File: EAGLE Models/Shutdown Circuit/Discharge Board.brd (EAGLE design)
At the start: 108 x 60 mm, 12 parts, among them U1 G2RL-1-E, U2 G2RL-1-E

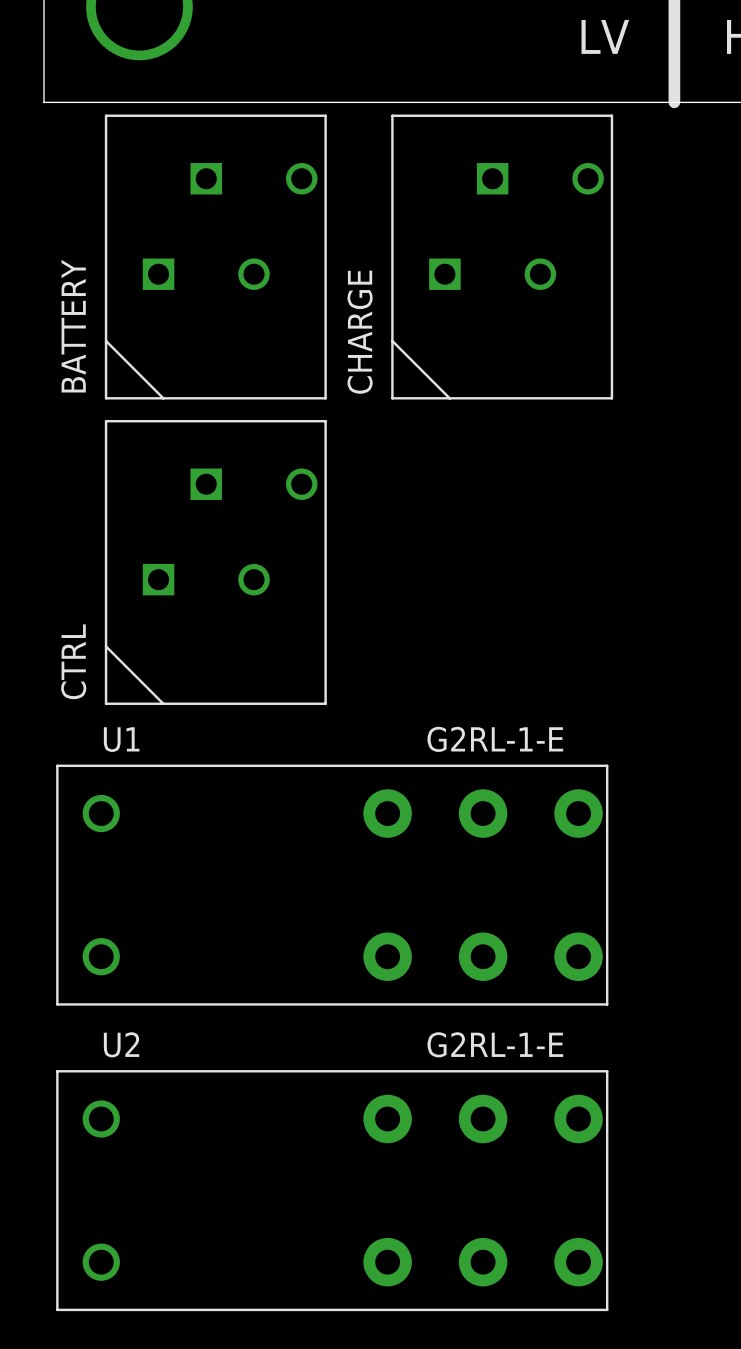
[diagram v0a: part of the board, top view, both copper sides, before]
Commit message: Deleted random parts that got added to the layout
These random parts were not in the schematic so I deleted them.
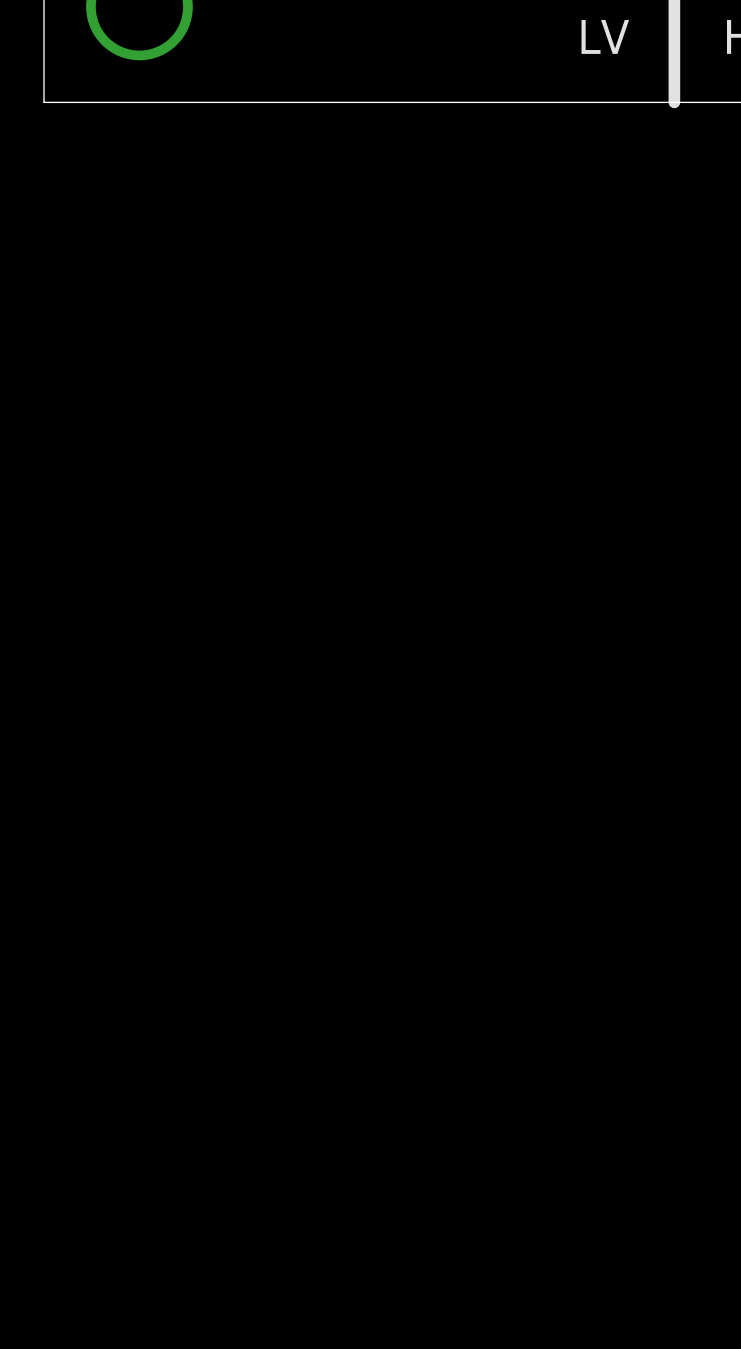
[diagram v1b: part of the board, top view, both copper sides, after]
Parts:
- removed BATTERY, CHARGE, CTRL: CONN_2, formula electric:CONNECTOR_2
- removed U1, U2: G2RL-1-E, formula electric:G2RL-1-E_RELAY
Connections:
- removed net N$1: CTRL.3, CTRL.4, U1.P$8, U2.P$8
- removed net N$12: BATTERY.1, BATTERY.2, U2.P$4, U2.P$5
- removed net N$13: BATTERY.3, BATTERY.4, U1.P$4, U1.P$5
- removed net N$14: CHARGE.1, CHARGE.2, U2.P$3, U2.P$6
- removed net N$15: CHARGE.3, CHARGE.4, U1.P$3, U1.P$6
- removed net N$2: CTRL.1, CTRL.2, U1.P$1, U2.P$1
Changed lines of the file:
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@@
 <?xml version="1.0" encoding="utf-8"?>
 <!DOCTYPE eagle SYSTEM "eagle.dtd">
-<eagle version="7.1.0">
+<eagle version="8.0.1">
 <drawing>
 <settings>
@@
 <element name="R2" library="formula electric" package="VISHAY_FS20W_RES" value="500" x="27" y="42"/>
 <element name="R3" library="formula electric" package="VISHAY_FS20W_RES" value="500" x="80" y="42" rot="R180"/>
-<element name="BATTERY" library="formula electric" package="CONNECTOR_2" value="CONN_2" x="6" y="-9"/>
-<element name="CTRL" library="formula electric" package="CONNECTOR_2" value="CONN_2" x="6" y="-25"/>
-<element name="U2" library="formula electric" package="G2RL-1-E_RELAY" value="G2RL-1-E" x="18" y="-57">
-<attribute name="COIL" value="DC 12" x="-13" y="-10" size="1.778" layer="27" display="off"/>
-</element>
-<element name="U1" library="formula electric" package="G2RL-1-E_RELAY" value="G2RL-1-E" x="18" y="-41">
-<attribute name="COIL" value="DC 12" x="-13" y="-26" size="1.778" layer="27" display="off"/>
-</element>
-<element name="CHARGE" library="formula electric" package="CONNECTOR_2" value="CONN_2" x="21" y="-9"/>
 </elements>
 <signals>
@@
 <wire x1="92.59" y1="51" x2="101.59" y2="42" width="5" layer="1"/>
 </signal>
-<signal name="N$1">
-<contactref element="CTRL" pad="4"/>
-<contactref element="CTRL" pad="3"/>
-<contactref element="U2" pad="P$8"/>
-<contactref element="U1" pad="P$8"/>
-<wire x1="3" y1="-37.25" x2="3" y2="-53.25" width="0" layer="19" extent="1-1"/>
-<wire x1="11" y1="-25" x2="3" y2="-37.25" width="0" layer="19" extent="1-1"/>
-<wire x1="13.5" y1="-20" x2="11" y2="-25" width="0" layer="19" extent="1-1"/>
-</signal>
-<signal name="N$2">
-<contactref element="CTRL" pad="2"/>
-<contactref element="CTRL" pad="1"/>
-<contactref element="U1" pad="P$1"/>
-<contactref element="U2" pad="P$1"/>
-<wire x1="3" y1="-44.75" x2="3" y2="-60.75" width="0" layer="19" extent="1-1"/>
-<wire x1="6" y1="-25" x2="3" y2="-44.75" width="0" layer="19" extent="1-1"/>
-<wire x1="8.5" y1="-20" x2="6" y2="-25" width="0" layer="19" extent="1-1"/>
-</signal>
-<signal name="N$12">
-<contactref element="BATTERY" pad="2"/>
-<contactref element="BATTERY" pad="1"/>
-<contactref element="U2" pad="P$5"/>
-<contactref element="U2" pad="P$4"/>
-<wire x1="28" y1="-53.25" x2="28" y2="-60.75" width="0" layer="19" extent="1-1"/>
-<wire x1="6" y1="-9" x2="28" y2="-53.25" width="0" layer="19" extent="1-1"/>
-<wire x1="8.5" y1="-4" x2="6" y2="-9" width="0" layer="19" extent="1-1"/>
-</signal>
-<signal name="N$13">
-<contactref element="BATTERY" pad="4"/>
-<contactref element="BATTERY" pad="3"/>
-<contactref element="U1" pad="P$5"/>
-<contactref element="U1" pad="P$4"/>
-<wire x1="28" y1="-37.25" x2="28" y2="-44.75" width="0" layer="19" extent="1-1"/>
-<wire x1="11" y1="-9" x2="28" y2="-37.25" width="0" layer="19" extent="1-1"/>
-<wire x1="13.5" y1="-4" x2="11" y2="-9" width="0" layer="19" extent="1-1"/>
-</signal>
-<signal name="N$14">
-<contactref element="CHARGE" pad="2"/>
-<contactref element="CHARGE" pad="1"/>
-<contactref element="U2" pad="P$6"/>
-<contactref element="U2" pad="P$3"/>
-<wire x1="23" y1="-53.25" x2="23" y2="-60.75" width="0" layer="19" extent="1-1"/>
-<wire x1="21" y1="-9" x2="23" y2="-53.25" width="0" layer="19" extent="1-1"/>
-<wire x1="23.5" y1="-4" x2="21" y2="-9" width="0" layer="19" extent="1-1"/>
-</signal>
-<signal name="N$15">
-<contactref element="CHARGE" pad="4"/>
-<contactref element="CHARGE" pad="3"/>
-<contactref element="U1" pad="P$6"/>
-<contactref element="U1" pad="P$3"/>
-<wire x1="26" y1="-9" x2="28.5" y2="-4" width="0" layer="19" extent="1-1"/>
-<wire x1="23" y1="-37.25" x2="26" y2="-9" width="0" layer="19" extent="1-1"/>
-<wire x1="23" y1="-44.75" x2="23" y2="-37.25" width="0" layer="19" extent="1-1"/>
-</signal>
 </signals>

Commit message: renamed trace to have better name
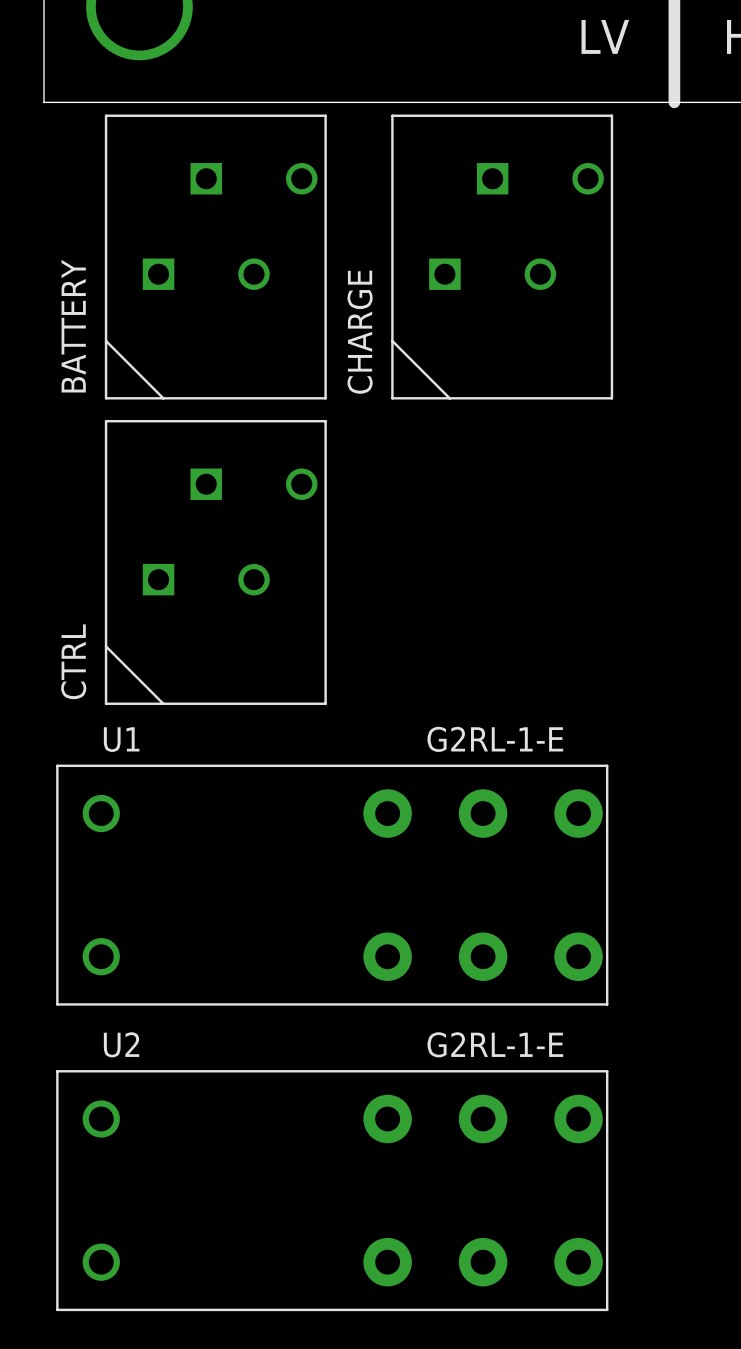
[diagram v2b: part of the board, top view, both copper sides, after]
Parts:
- added BATTERY, CHARGE, CTRL: CONN_2, formula electric:CONNECTOR_2
- added U1, U2: G2RL-1-E, formula electric:G2RL-1-E_RELAY
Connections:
- new net N$1: CTRL.3, CTRL.4, U1.P$8, U2.P$8
- new net N$12: BATTERY.1, BATTERY.2, U2.P$4, U2.P$5
- new net N$13: BATTERY.3, BATTERY.4, U1.P$4, U1.P$5
- new net N$14: CHARGE.1, CHARGE.2, U2.P$3, U2.P$6
- new net N$15: CHARGE.3, CHARGE.4, U1.P$3, U1.P$6
- new net N$2: CTRL.1, CTRL.2, U1.P$1, U2.P$1
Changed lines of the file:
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@@
 <?xml version="1.0" encoding="utf-8"?>
 <!DOCTYPE eagle SYSTEM "eagle.dtd">
-<eagle version="8.0.1">
+<eagle version="7.1.0">
 <drawing>
 <settings>
@@
 <element name="R2" library="formula electric" package="VISHAY_FS20W_RES" value="500" x="27" y="42"/>
 <element name="R3" library="formula electric" package="VISHAY_FS20W_RES" value="500" x="80" y="42" rot="R180"/>
+<element name="BATTERY" library="formula electric" package="CONNECTOR_2" value="CONN_2" x="6" y="-9"/>
+<element name="CTRL" library="formula electric" package="CONNECTOR_2" value="CONN_2" x="6" y="-25"/>
+<element name="U2" library="formula electric" package="G2RL-1-E_RELAY" value="G2RL-1-E" x="18" y="-57">
+<attribute name="COIL" value="DC 12" x="-13" y="-10" size="1.778" layer="27" display="off"/>
+</element>
+<element name="U1" library="formula electric" package="G2RL-1-E_RELAY" value="G2RL-1-E" x="18" y="-41">
+<attribute name="COIL" value="DC 12" x="-13" y="-26" size="1.778" layer="27" display="off"/>
+</element>
+<element name="CHARGE" library="formula electric" package="CONNECTOR_2" value="CONN_2" x="21" y="-9"/>
 </elements>
 <signals>
@@
 <wire x1="92.59" y1="51" x2="101.59" y2="42" width="5" layer="1"/>
 </signal>
+<signal name="N$1">
+<contactref element="CTRL" pad="4"/>
+<contactref element="CTRL" pad="3"/>
+<contactref element="U2" pad="P$8"/>
+<contactref element="U1" pad="P$8"/>
+<wire x1="3" y1="-37.25" x2="3" y2="-53.25" width="0" layer="19" extent="1-1"/>
+<wire x1="11" y1="-25" x2="3" y2="-37.25" width="0" layer="19" extent="1-1"/>
+<wire x1="13.5" y1="-20" x2="11" y2="-25" width="0" layer="19" extent="1-1"/>
+</signal>
+<signal name="N$2">
+<contactref element="CTRL" pad="2"/>
+<contactref element="CTRL" pad="1"/>
+<contactref element="U1" pad="P$1"/>
+<contactref element="U2" pad="P$1"/>
+<wire x1="3" y1="-44.75" x2="3" y2="-60.75" width="0" layer="19" extent="1-1"/>
+<wire x1="6" y1="-25" x2="3" y2="-44.75" width="0" layer="19" extent="1-1"/>
+<wire x1="8.5" y1="-20" x2="6" y2="-25" width="0" layer="19" extent="1-1"/>
+</signal>
+<signal name="N$12">
+<contactref element="BATTERY" pad="2"/>
+<contactref element="BATTERY" pad="1"/>
+<contactref element="U2" pad="P$5"/>
+<contactref element="U2" pad="P$4"/>
+<wire x1="28" y1="-53.25" x2="28" y2="-60.75" width="0" layer="19" extent="1-1"/>
+<wire x1="6" y1="-9" x2="28" y2="-53.25" width="0" layer="19" extent="1-1"/>
+<wire x1="8.5" y1="-4" x2="6" y2="-9" width="0" layer="19" extent="1-1"/>
+</signal>
+<signal name="N$13">
+<contactref element="BATTERY" pad="4"/>
+<contactref element="BATTERY" pad="3"/>
+<contactref element="U1" pad="P$5"/>
+<contactref element="U1" pad="P$4"/>
+<wire x1="28" y1="-37.25" x2="28" y2="-44.75" width="0" layer="19" extent="1-1"/>
+<wire x1="11" y1="-9" x2="28" y2="-37.25" width="0" layer="19" extent="1-1"/>
+<wire x1="13.5" y1="-4" x2="11" y2="-9" width="0" layer="19" extent="1-1"/>
+</signal>
+<signal name="N$14">
+<contactref element="CHARGE" pad="2"/>
+<contactref element="CHARGE" pad="1"/>
+<contactref element="U2" pad="P$6"/>
+<contactref element="U2" pad="P$3"/>
+<wire x1="23" y1="-53.25" x2="23" y2="-60.75" width="0" layer="19" extent="1-1"/>
+<wire x1="21" y1="-9" x2="23" y2="-53.25" width="0" layer="19" extent="1-1"/>
+<wire x1="23.5" y1="-4" x2="21" y2="-9" width="0" layer="19" extent="1-1"/>
+</signal>
+<signal name="N$15">
+<contactref element="CHARGE" pad="4"/>
+<contactref element="CHARGE" pad="3"/>
+<contactref element="U1" pad="P$6"/>
+<contactref element="U1" pad="P$3"/>
+<wire x1="26" y1="-9" x2="28.5" y2="-4" width="0" layer="19" extent="1-1"/>
+<wire x1="23" y1="-37.25" x2="26" y2="-9" width="0" layer="19" extent="1-1"/>
+<wire x1="23" y1="-44.75" x2="23" y2="-37.25" width="0" layer="19" extent="1-1"/>
+</signal>
 </signals>
